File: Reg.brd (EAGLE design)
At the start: 25.4 x 21 mm, 13 parts, among them Q1 NPN2SC3422-2, Q2 NPN2SC3325, Q3 PNP2SA1313, Q4 NPN2SC3325

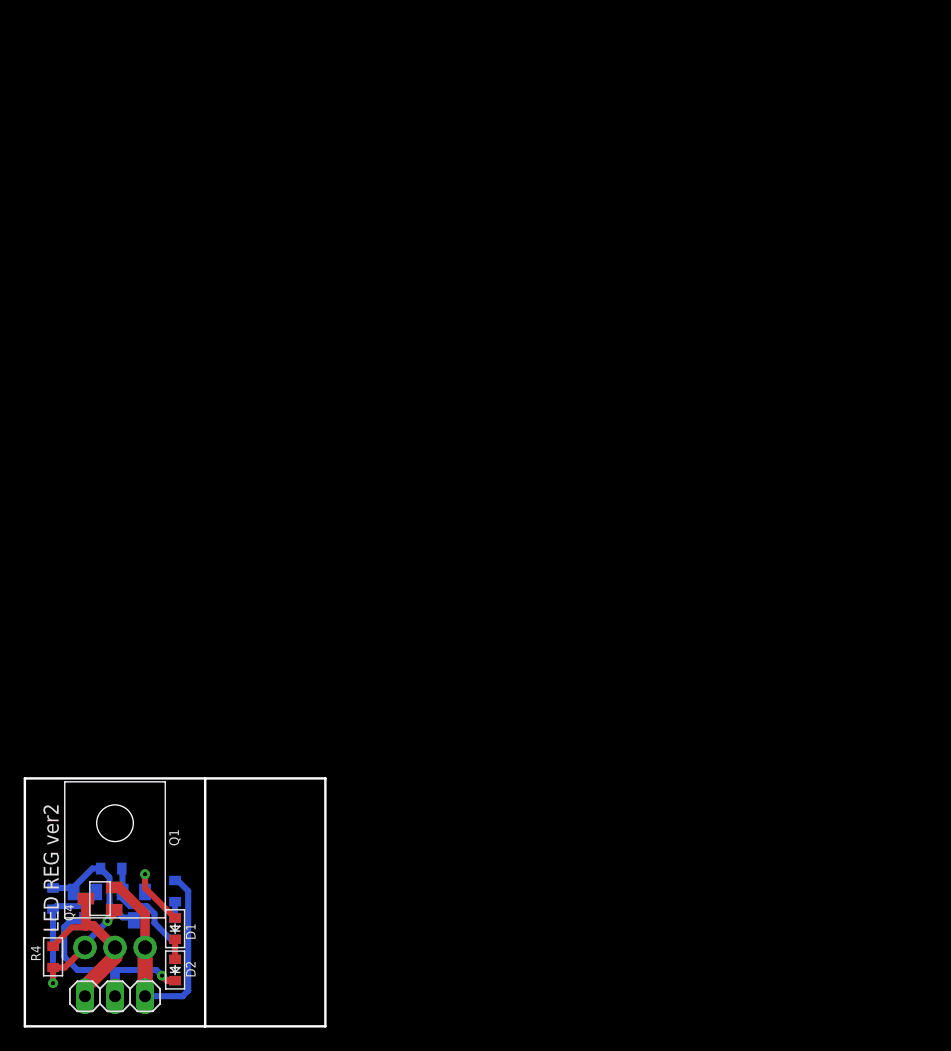
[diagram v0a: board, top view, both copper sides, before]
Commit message: Vカット
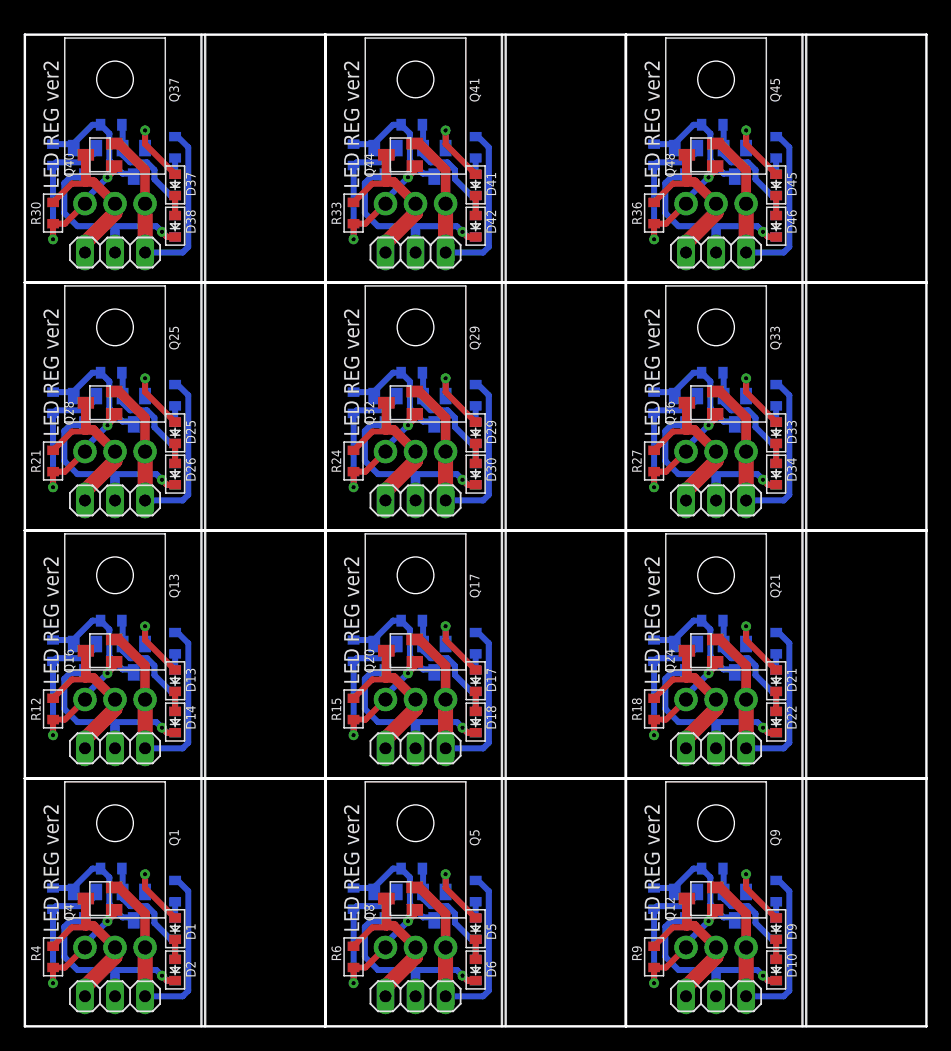
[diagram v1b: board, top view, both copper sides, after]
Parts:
- added C1, C10, C11, C12, C2, C3, C4, C5, C6, C8, C9: 100p, my_rcl:1608
- added D10, D13, D14, D17, D18, D21, D22, D25, D26, D29, D30, D33, D34, D37, D38, D41, D42, D45, D46, D5, D6, D9: SHORT, my_rcl:D1608
- added D11, D12, D15, D16, D19, D20, D23, D24, D27, D28, D31, D32, D35, D36, D39, D40, D43, D44, D47, D48, D7, D8: BLUE, my_rcl:D1608
- added JP10, JP11, JP12, JP2, JP3, JP4, JP5, JP6, JP7, JP8, JP9: CON, pinhead:1X03
- added Q10, Q12, Q14, Q16, Q18, Q20, Q22, Q24, Q26, Q28, Q30, Q32, Q34, Q36, Q38, Q40, Q42, Q44, Q46, Q48, Q6, Q8: NPN2SC3325, my_ic:SC59
- added Q11, Q15, Q19, Q23, Q27, Q31, Q35, Q39, Q43, Q47, Q7: PNP2SA1313, my_ic:SC59
- added Q13, Q17, Q21, Q25, Q29, Q33, Q37, Q41, Q45, Q5, Q9: NPN2SC3422-2, my_ic:TO126-2
- added R10, R11, R12, R13, R14, R15, R16, R17, R18, R19, R20, R21, R22, R23, R24, R25, R26, R27, R28, R29, R3, R30, R31, R32, R33, R34, R35, R36, R5, R6, R7, R8, R9: 1.5k, my_rcl:1608
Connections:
- new net GND1: D6.K, JP2.2, Q7.3, R3.1
- new net GND10: D42.K, JP11.2, Q43.3, R31.1
- new net GND11: D46.K, JP12.2, Q47.3, R34.1
- new net GND2: D10.K, JP3.2, Q11.3, R7.1
- new net GND3: D14.K, JP4.2, Q15.3, R10.1
- new net GND4: D18.K, JP5.2, Q19.3, R13.1
- new net GND5: D22.K, JP6.2, Q23.3, R16.1
- new net GND6: D26.K, JP7.2, Q27.3, R19.1
- new net GND7: D30.K, JP8.2, Q31.3, R22.1
- new net GND8: D34.K, JP9.2, Q35.3, R25.1
- new net GND9: D38.K, JP10.2, Q39.3, R28.1
- new net IN1: JP2.1, Q5.2, Q8.3, R6.2
- new net IN10: JP11.1, Q41.2, Q44.3, R33.2
- new net IN11: JP12.1, Q45.2, Q48.3, R36.2
- new net IN2: JP3.1, Q12.3, Q9.2, R9.2
- new net IN3: JP4.1, Q13.2, Q16.3, R12.2
- new net IN4: JP5.1, Q17.2, Q20.3, R15.2
- new net IN5: JP6.1, Q21.2, Q24.3, R18.2
- new net IN6: JP7.1, Q25.2, Q28.3, R21.2
- new net IN7: JP8.1, Q29.2, Q32.3, R24.2
- new net IN8: JP9.1, Q33.2, Q36.3, R27.2
- new net IN9: JP10.1, Q37.2, Q40.3, R30.2
- new net N$11: C1.1, Q6.3, Q7.1, R5.1
- new net N$12: D7.A, D8.K
- new net N$13: C2.2, D11.K, Q10.1, R7.2
- new net N$14: D10.A, D9.K
- new net N$15: D9.A, Q10.2
- new net N$16: Q11.2, Q12.1, Q9.3, R8.2, R9.1
- new net N$17: C2.1, Q10.3, Q11.1, R8.1
- new net N$18: D11.A, D12.K
- new net N$19: C3.2, D15.K, Q14.1, R10.2
- new net N$20: D13.K, D14.A
- new net N$21: D13.A, Q14.2
- new net N$22: Q13.3, Q15.2, Q16.1, R11.2, R12.1
- new net N$23: C3.1, Q14.3, Q15.1, R11.1
- new net N$24: D15.A, D16.K
- new net N$25: C4.2, D19.K, Q18.1, R13.2
- new net N$26: D17.K, D18.A
- new net N$27: D17.A, Q18.2
- new net N$28: Q17.3, Q19.2, Q20.1, R14.2, R15.1
- new net N$29: C4.1, Q18.3, Q19.1, R14.1
- new net N$30: D19.A, D20.K
- new net N$31: C5.2, D23.K, Q22.1, R16.2
- new net N$32: D21.K, D22.A
- new net N$33: D21.A, Q22.2
- new net N$34: Q21.3, Q23.2, Q24.1, R17.2, R18.1
- new net N$35: C5.1, Q22.3, Q23.1, R17.1
- new net N$36: D23.A, D24.K
- new net N$37: C6.2, D27.K, Q26.1, R19.2
- new net N$38: D25.K, D26.A
- new net N$39: D25.A, Q26.2
- new net N$40: Q25.3, Q27.2, Q28.1, R20.2, R21.1
- new net N$41: C6.1, Q26.3, Q27.1, R20.1
- new net N$42: D27.A, D28.K
- new net N$43: C8.2, D31.K, Q30.1, R22.2
- new net N$44: D29.K, D30.A
- new net N$45: D29.A, Q30.2
- new net N$46: Q29.3, Q31.2, Q32.1, R23.2, R24.1
- new net N$47: C8.1, Q30.3, Q31.1, R23.1
- new net N$48: D31.A, D32.K
- new net N$49: C9.2, D35.K, Q34.1, R25.2
- new net N$50: D33.K, D34.A
- new net N$51: D33.A, Q34.2
- new net N$52: Q33.3, Q35.2, Q36.1, R26.2, R27.1
- new net N$53: C9.1, Q34.3, Q35.1, R26.1
- new net N$54: D35.A, D36.K
- new net N$55: C10.2, D39.K, Q38.1, R28.2
- new net N$56: D37.K, D38.A
- new net N$57: D37.A, Q38.2
- new net N$58: Q37.3, Q39.2, Q40.1, R29.2, R30.1
- new net N$59: C10.1, Q38.3, Q39.1, R29.1
- new net N$6: C1.2, D7.K, Q6.1, R3.2
- new net N$60: D39.A, D40.K
- new net N$61: C11.2, D43.K, Q42.1, R31.2
- new net N$62: D41.K, D42.A
- new net N$63: D41.A, Q42.2
- new net N$64: Q41.3, Q43.2, Q44.1, R32.2, R33.1
- new net N$65: C11.1, Q42.3, Q43.1, R32.1
- new net N$66: D43.A, D44.K
- new net N$67: C12.2, D47.K, Q46.1, R34.2
- new net N$68: D45.K, D46.A
- new net N$69: D45.A, Q46.2
- new net N$7: D5.K, D6.A
- new net N$70: Q45.3, Q47.2, Q48.1, R35.2, R36.1
- new net N$71: C12.1, Q46.3, Q47.1, R35.1
- new net N$72: D47.A, D48.K
- new net N$8: D5.A, Q6.2
- new net N$9: Q5.3, Q7.2, Q8.1, R5.2, R6.1
- new net OUT1: D8.A, JP2.3, Q5.1, Q8.2
- new net OUT10: D44.A, JP11.3, Q41.1, Q44.2
- new net OUT11: D48.A, JP12.3, Q45.1, Q48.2
- new net OUT2: D12.A, JP3.3, Q12.2, Q9.1
- new net OUT3: D16.A, JP4.3, Q13.1, Q16.2
- new net OUT4: D20.A, JP5.3, Q17.1, Q20.2
- new net OUT5: D24.A, JP6.3, Q21.1, Q24.2
- new net OUT6: D28.A, JP7.3, Q25.1, Q28.2
- new net OUT7: D32.A, JP8.3, Q29.1, Q32.2
- new net OUT8: D36.A, JP9.3, Q33.1, Q36.2
- new net OUT9: D40.A, JP10.3, Q37.1, Q40.2
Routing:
- net OUT9: track 0.00 -> 24.3 mm
- net OUT6: track 0.00 -> 24.3 mm
- net OUT3: track 0.00 -> 24.3 mm
- net OUT8: track 0.00 -> 24.3 mm
- net OUT7: track 0.00 -> 24.3 mm
- net OUT5: track 0.00 -> 24.3 mm
- net OUT2: track 0.00 -> 24.3 mm
- net OUT11: track 0.00 -> 24.3 mm
- net OUT1: track 0.00 -> 24.3 mm
- net OUT4: track 0.00 -> 24.3 mm
- net OUT10: track 0.00 -> 24.3 mm
- net N$52: track 0.00 -> 19.6 mm, vias 0 -> 2
- net N$34: track 0.00 -> 19.6 mm, vias 0 -> 2
- net N$28: track 0.00 -> 19.6 mm, vias 0 -> 2
- net N$16: track 0.00 -> 19.6 mm, vias 0 -> 2
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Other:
- board size 25.4 x 21 mm -> 76.2 x 83.8 mm
- board text added: "C7"
- board text added: "D1"
- board text added: "D2"
- board text added: "D3"
- board text added: "D4"
- board text added: "Q1"
- board text added: "Q2"
- board text added: "Q3"
- board text added: "Q4"
- board text added: "R1"
- board text added: "R2"
- board text added: "R4"
